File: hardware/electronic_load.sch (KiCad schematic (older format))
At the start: 27 parts, among them J1 Screw_Terminal_01x02, J2 SPI, J3 UART, P1 Power connector, P2 LCD, P3 One Wire, SW2 Back, SW3 Down, SW4 Up, SW5 Enter, U8 FDV303N

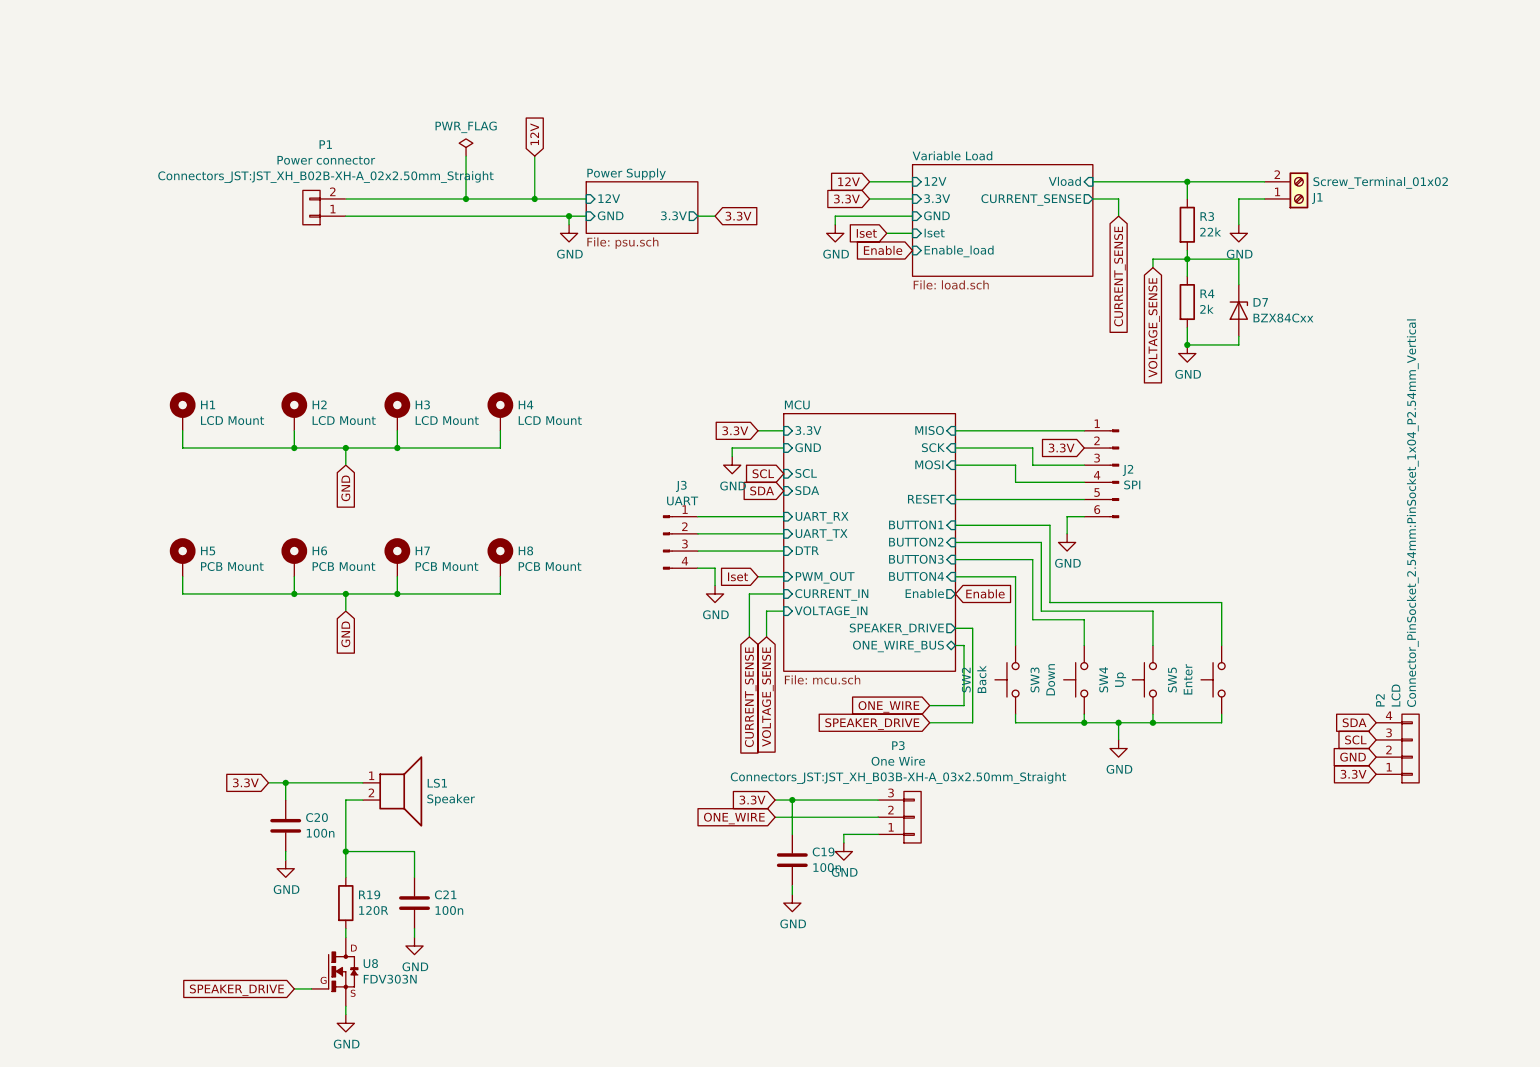
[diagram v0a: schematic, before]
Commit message: Blebleble
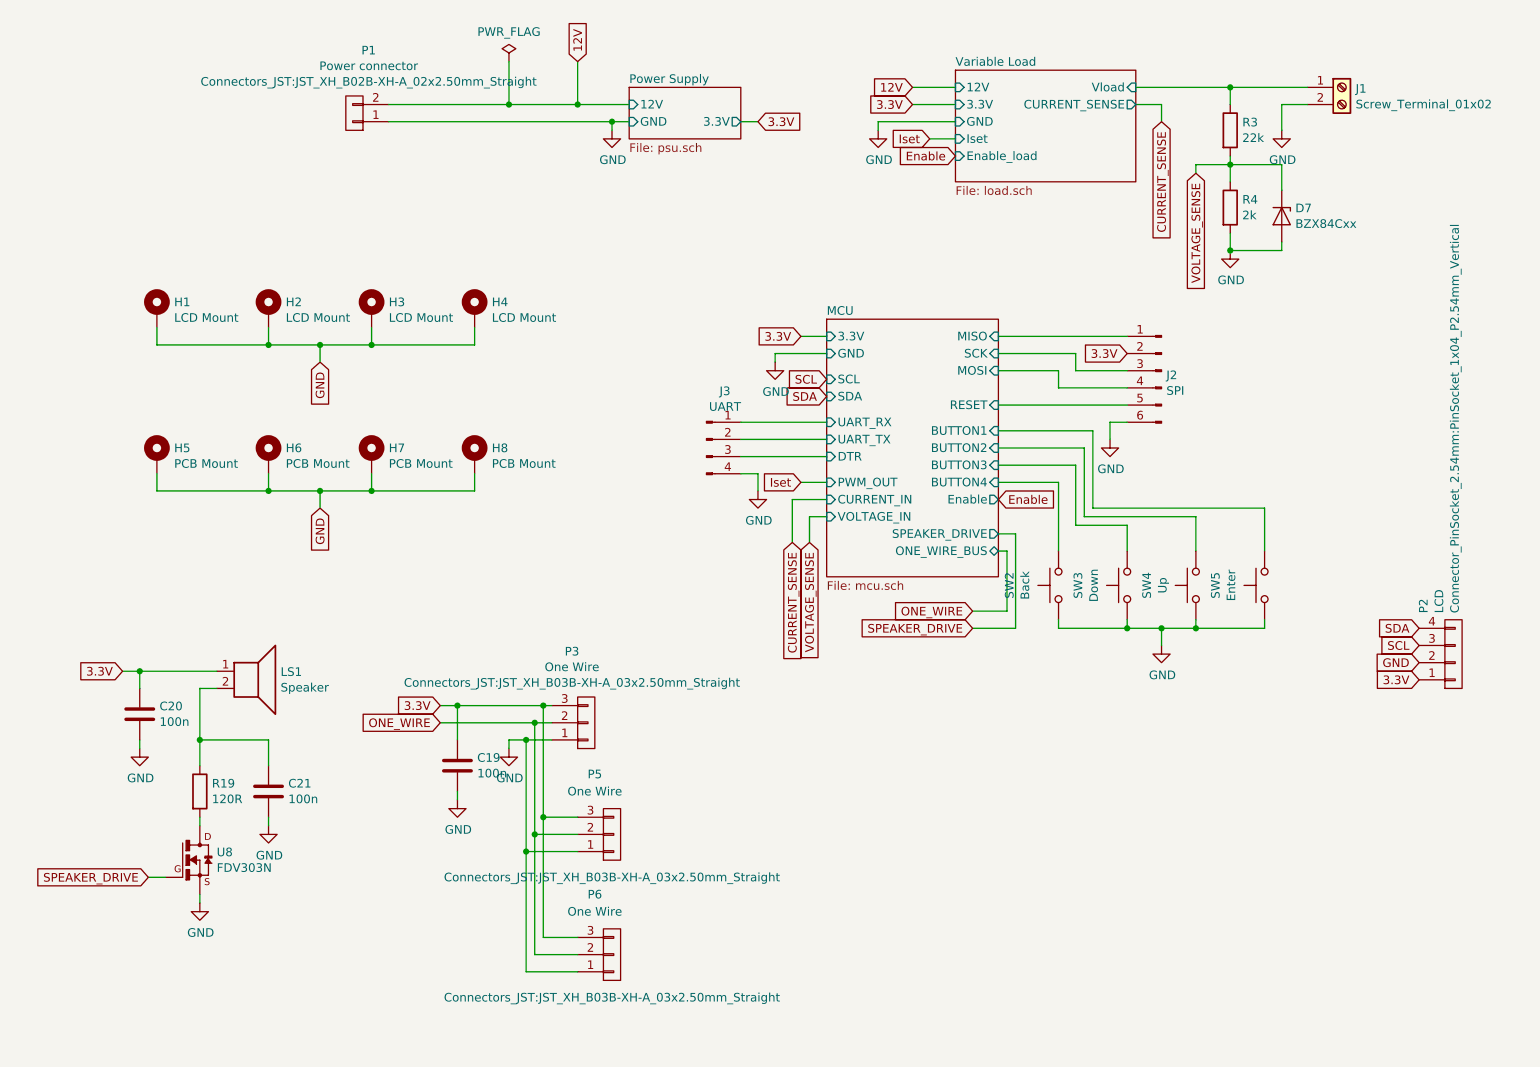
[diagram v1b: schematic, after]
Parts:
- added P5, P6: One Wire, Connectors_JST:JST_XH_B03B-XH-A_03x2.50mm_Straight, symbol conn:CONN_01X03
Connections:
- net 3.3V: now also P5.3 (P3), P6.3 (P3)
- net GND: now also J1.2 (Pin_2), P5.1 (P1), P6.1 (P1); no longer J1.1 (Pin_1)
- net ONE_WIRE: now also P5.2 (P2), P6.2 (P2)
- net Variable Load/Vload: now also J1.1 (Pin_1); no longer J1.2 (Pin_2)
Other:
- moved on the sheet: C19, C20, C21, D7, H1, H2, H3, H4, H5, H6, H7, H8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
